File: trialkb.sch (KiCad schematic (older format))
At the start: 24 parts, among them SW1 SW_Push, U1 ATmega32U4-AU, Y1 16MHz

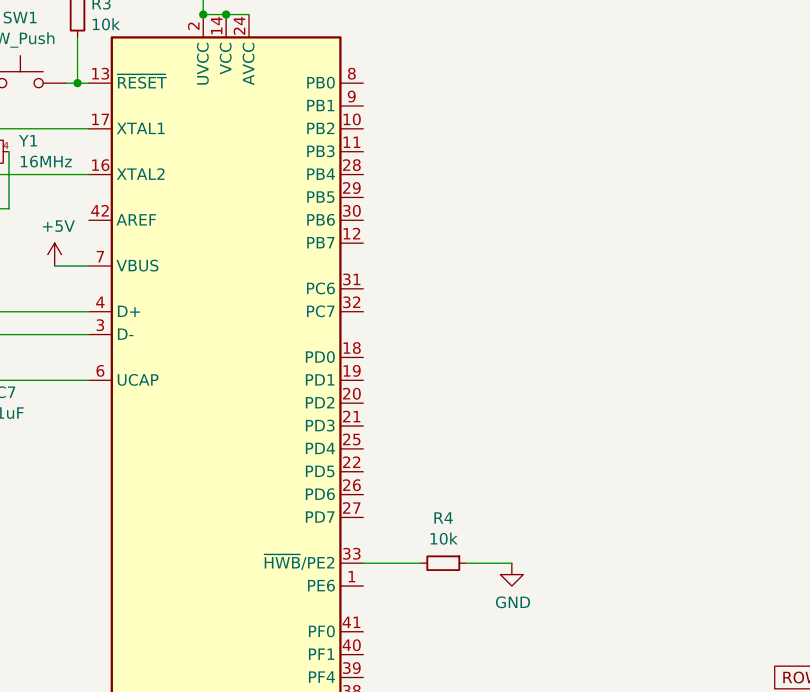
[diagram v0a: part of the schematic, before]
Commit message: routing complete
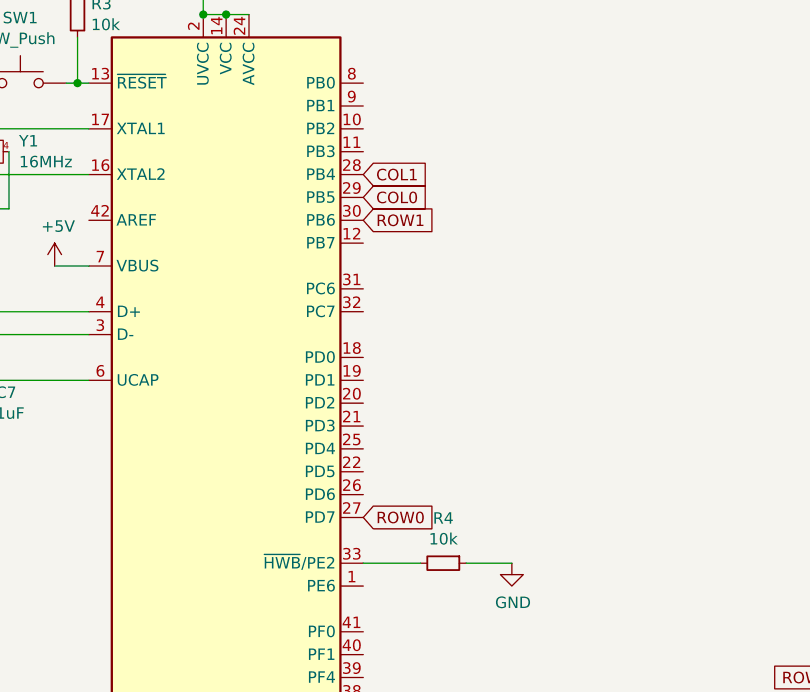
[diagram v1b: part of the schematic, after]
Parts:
- SW1: footprint random-keyboard-parts:Reset_Pretty -> random-keyboard-parts:SKQG-1155865
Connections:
- net COL0: now also U1.29 (PB5)
- net COL1: now also U1.28 (PB4)
- net ROW0: now also U1.27 (PD7)
- net ROW1: now also U1.30 (PB6)
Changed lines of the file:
@@
 F 0 "SW1" H 3650 2385 50  0000 C CNN
 F 1 "SW_Push" H 3650 2294 50  0000 C CNN
-F 2 "random-keyboard-parts:Reset_Pretty" H 3650 2300 50  0001 C CNN
+F 2 "random-keyboard-parts:SKQG-1155865" H 3650 2300 50  0001 C CNN
 F 3 "~" H 3650 2300 50  0001 C CNN
 	1    3650 2100
@@
 ROW1
 Connection ~ 8400 1850
+Text GLabel 5150 2500 2    50   Input ~ 0
+COL1
+Text GLabel 5150 2600 2    50   Input ~ 0
+COL0
+Text GLabel 5150 2700 2    50   Input ~ 0
+ROW1
+Text GLabel 5150 4000 2    50   Input ~ 0
+ROW0
 $EndSCHEMATC
